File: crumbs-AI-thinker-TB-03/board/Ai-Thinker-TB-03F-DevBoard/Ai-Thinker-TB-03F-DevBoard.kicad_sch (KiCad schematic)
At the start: 8 parts, among them J1 USB_C_Receptacle_PowerOnly_6P, J2 Conn_01x15, SW1 SW_Push_Width_Bit_Smaller_Tha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, U1 CH340C, U2 AI_Thinker_TB-03F, U3 AMS1117-3.3

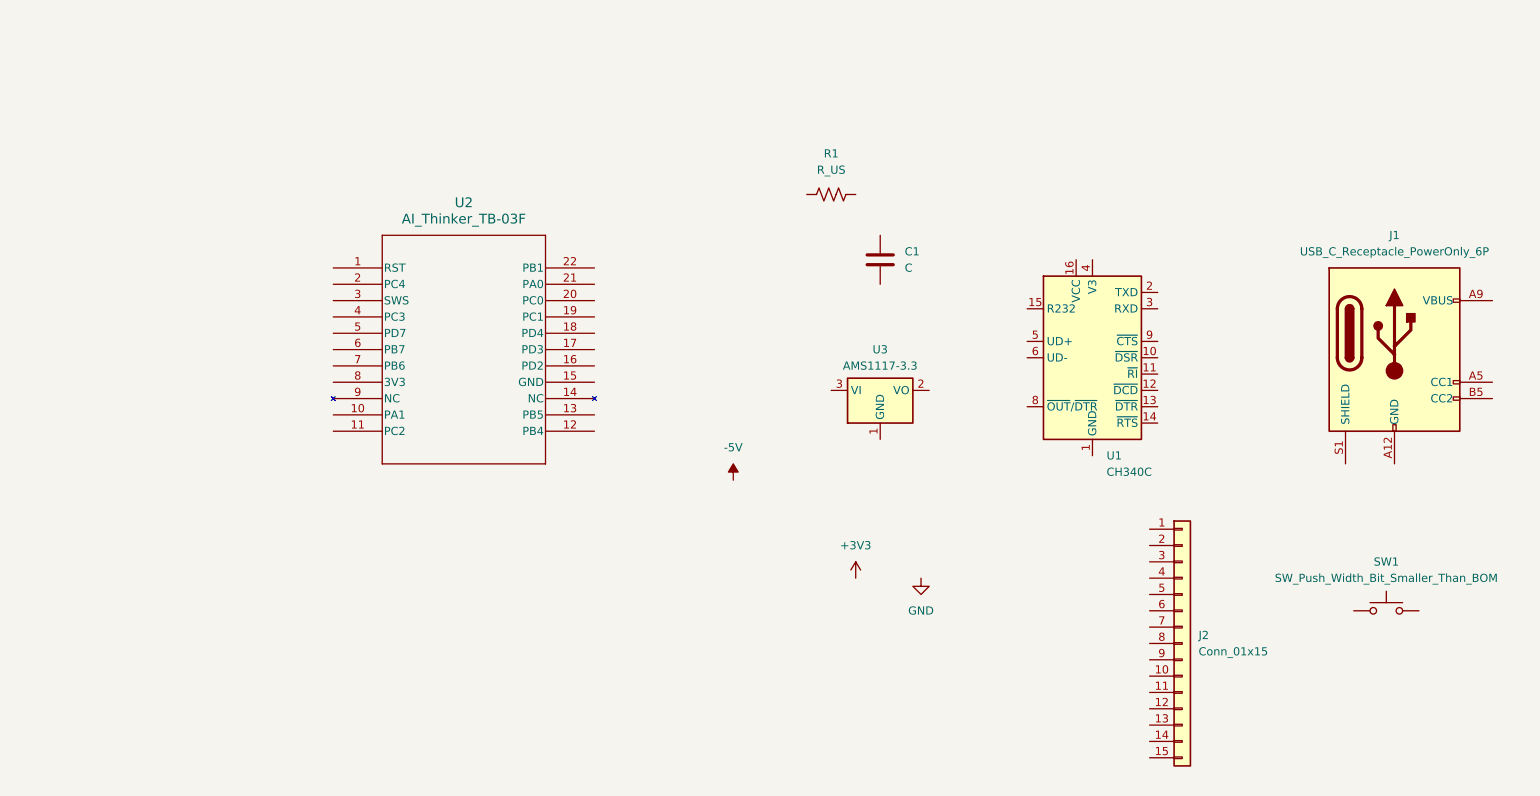
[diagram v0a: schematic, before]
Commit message: [12-09-2005] TB-03 Finish Schematic, need recheck
add readme

Update README.md
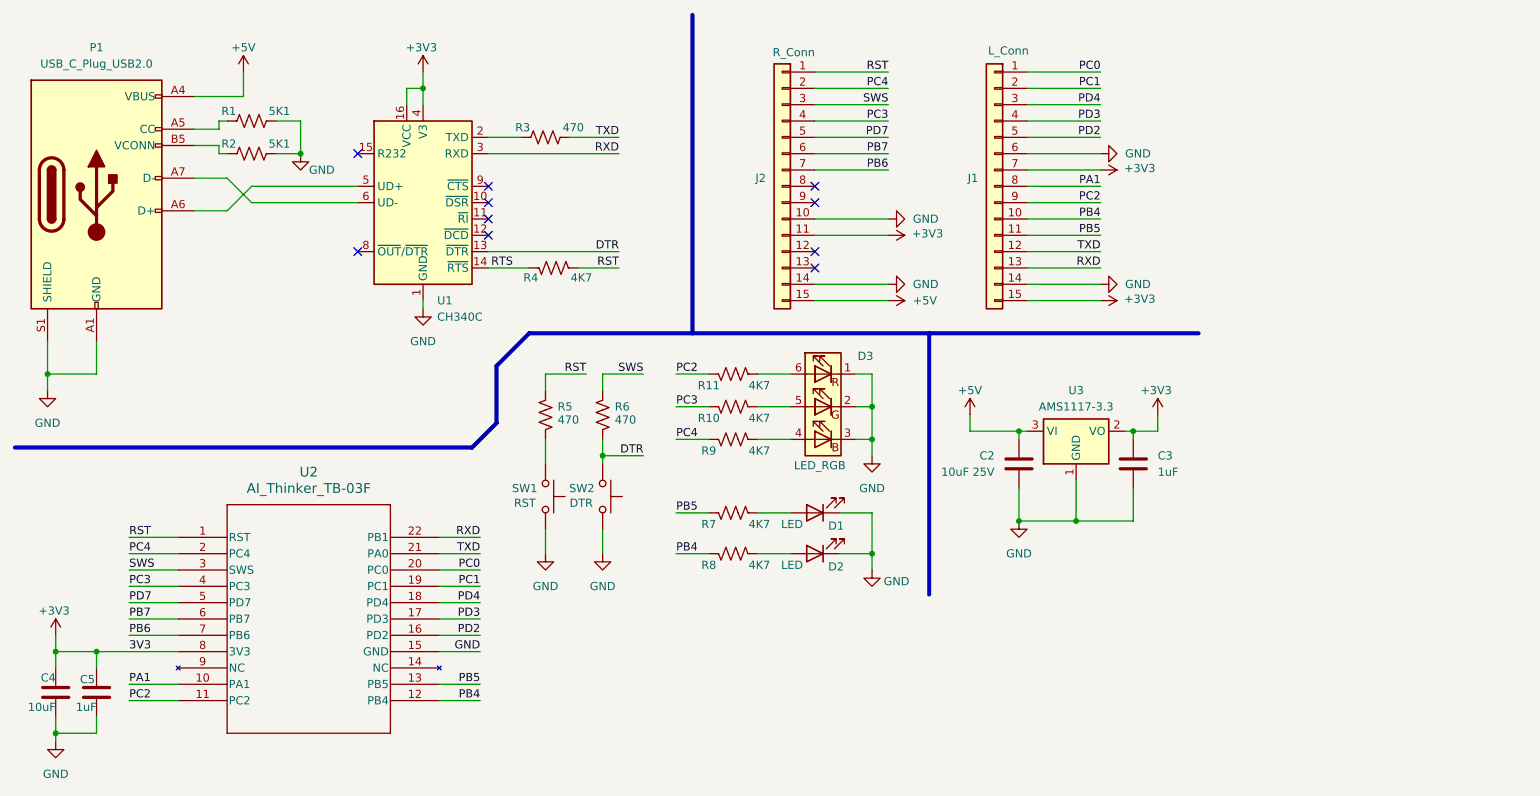
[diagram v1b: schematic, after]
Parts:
- removed C1: C, symbol Device:C
- removed J1: USB_C_Receptacle_PowerOnly_6P, Connector_USB:USB_C_Receptacle_GCT_USB4135-GF-A_6P_TopMnt_Horizontal, symbol Connector:USB_C_Receptacle_PowerOnly_6P
- added C2: 10uF 25V, symbol Device:C
- added C3, C5: 1uF, symbol Device:C
- added C4: 10uF, symbol Device:C
- added D1, D2: LED, symbol Device:LED
- added D3: LED_RGB, LED_SMD:LED_WS2812_PLCC6_5.0x5.0mm_P1.6mm, symbol Device:LED_RGB
- added J1: L_Conn, Connector_PinHeader_2.54mm:PinHeader_1x15_P2.54mm_Vertical, symbol Connector_Generic:Conn_01x15
- added P1: USB_C_Plug_USB2.0, Connector_USB:USB_C_Receptacle_XKB_U262-16XN-4BVC11, symbol Connector:USB_C_Plug_USB2.0
- added R10, R11, R4, R7, R8, R9: 4K7, symbol Device:R_US
- added R2: 5K1, symbol Device:R_US
- added R3, R5, R6: 470, symbol Device:R_US
- added SW2: DTR, Button_Switch_SMD:SW_SPST_EVQPE1, symbol Switch:SW_Push
- J2: value Conn_01x15 -> R_Conn
- R1: value R_US -> 5K1
- SW1: value SW_Push_Width_Bit_Smaller_Than_BOM -> RST
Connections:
- net +3V3: now also J2.11 (Pin_11), U1.16 (VCC), U1.4 (V3), U2.8 (3V3), U3.2 (VO), C3.1, C4.1, C5.1, J1.15 (Pin_15), J1.7 (Pin_7)
- net GND: now also J2.10 (Pin_10), J2.14 (Pin_14), R1.1, SW1.1, U1.1 (GND), U2.15 (GND), U3.1 (GND), C2.2, C3.2, C4.2, C5.2, D1.1 (K), D2.1 (K), D3.1 (RK), D3.2 (GK), D3.3 (BK), J1.14 (Pin_14), J1.6 (Pin_6), P1.A1 (GND), P1.A12 (GND), P1.B1 (GND), P1.B12 (GND), P1.S1 (SHIELD), R2.1, SW2.1
- net RST: now reaches J2.1 (Pin_1)
- net RST: now also U2.1 (RST), R4.1, R5.1
- net +5V: now reaches J2.15 (Pin_15)
- net +5V: now also U3.3 (VI), C2.1, P1.A4 (VBUS), P1.A9 (VBUS), P1.B4 (VBUS), P1.B9 (VBUS)
- net PC4: now reaches J2.2 (Pin_2)
- net PC4: now also U2.2 (PC4), R9.2
- net SWS: now reaches J2.3 (Pin_3)
- net SWS: now also U2.3 (SWS), R6.1
- net PC3: now reaches J2.4 (Pin_4)
- net PC3: now also U2.4 (PC3), R10.2
- net PD7: now reaches J2.5 (Pin_5)
- net PD7: now also U2.5 (PD7)
- net PB7: now reaches J2.6 (Pin_6)
- net PB7: now also U2.6 (PB7)
- net PB6: now reaches J2.7 (Pin_7)
- net PB6: now also U2.7 (PB6)
- net at SW1.2: now also R5.2
- net PA1: now reaches U2.10 (PA1)
- net PA1: now also J1.8 (Pin_8)
- net PC2: now reaches U2.11 (PC2)
- net PC2: now also J1.9 (Pin_9), R11.2
- net PB4: now reaches U2.12 (PB4)
- net PB4: now also J1.10 (Pin_10), R8.2
- net PB5: now reaches U2.13 (PB5)
- net PB5: now also J1.11 (Pin_11), R7.2
- net PD2: now reaches U2.16 (PD2)
- net PD2: now also J1.5 (Pin_5)
- net PD3: now reaches U2.17 (PD3)
- net PD3: now also J1.4 (Pin_4)
- net PD4: now reaches U2.18 (PD4)
- net PD4: now also J1.3 (Pin_3)
- net PC1: now reaches U2.19 (PC1)
- net PC1: now also J1.2 (Pin_2)
- net PC0: now reaches U2.20 (PC0)
- net PC0: now also J1.1 (Pin_1)
- net TXD: now reaches U2.21 (PA0)
- net TXD: now also J1.12 (Pin_12), R3.1
- net RXD: now reaches U2.22 (PB1)
- net RXD: now also U1.3 (RXD), J1.13 (Pin_13)
- net at R1.2: now also P1.A5 (CC)
- net DTR: now reaches U1.13 (~{DTR})
- net DTR: now also R6.2, SW2.2
- net RTS: now reaches U1.14 (~{RTS})
- net RTS: now also R4.2
- net at U1.2 (TXD): now also R3.2
- net at U1.5 (UD+): now also P1.A6 (D+)
- net at U1.6 (UD-): now also P1.A7 (D-)
- new net: D3.6 (RA), R11.1
- new net: D1.2 (A), R7.1
- new net: P1.B5 (VCONN), R2.2
- new net: D3.5 (GA), R10.1
- new net: D2.2 (A), R8.1
- new net: D3.4 (BA), R9.1
- no-connect marks 0 -> 10
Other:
- title: (none) -> AI Thinker TB-03F Dev Board
- moved on the sheet: J2, U2, U3
